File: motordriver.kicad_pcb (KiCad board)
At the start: 2 copper layers, 8 parts, among them J1 power terminal, J2 motor A, J3 motor B, J4 control pins, U1 L7805, U2 L293D

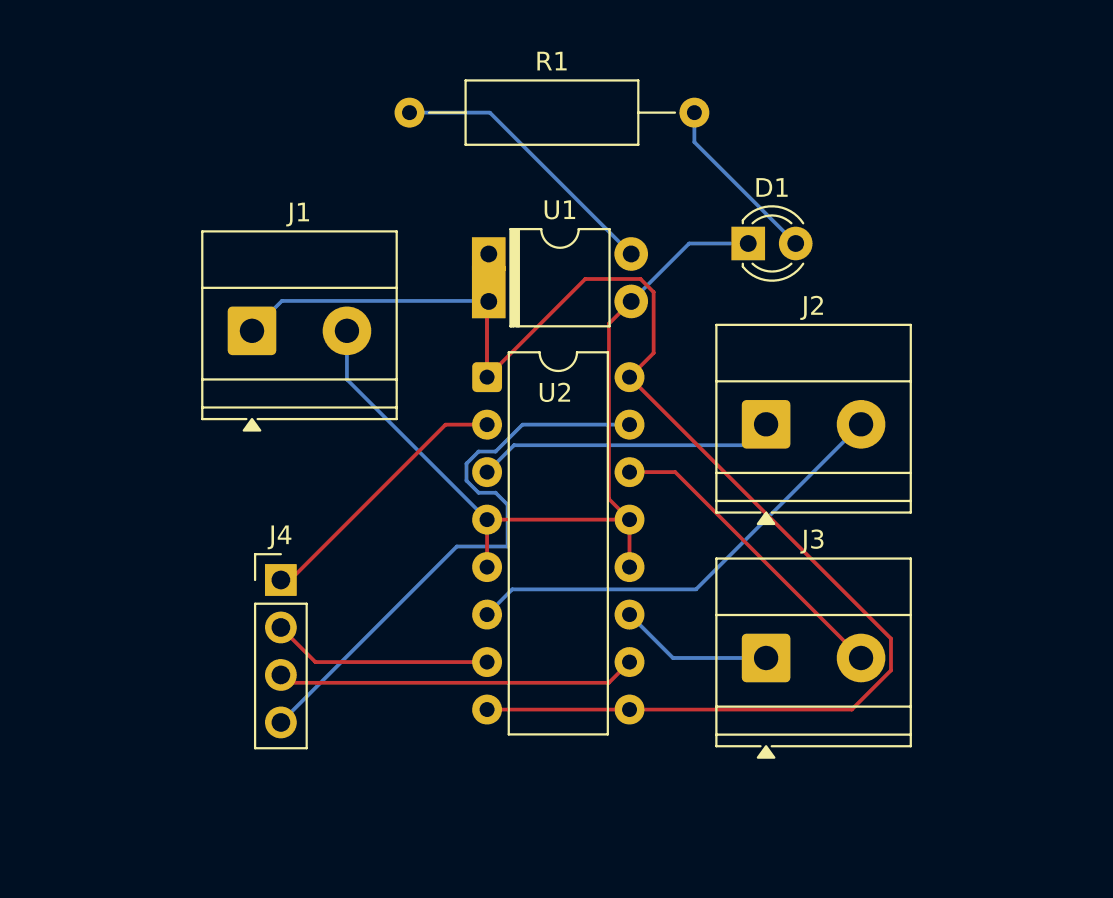
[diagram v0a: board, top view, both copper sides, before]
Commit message: done
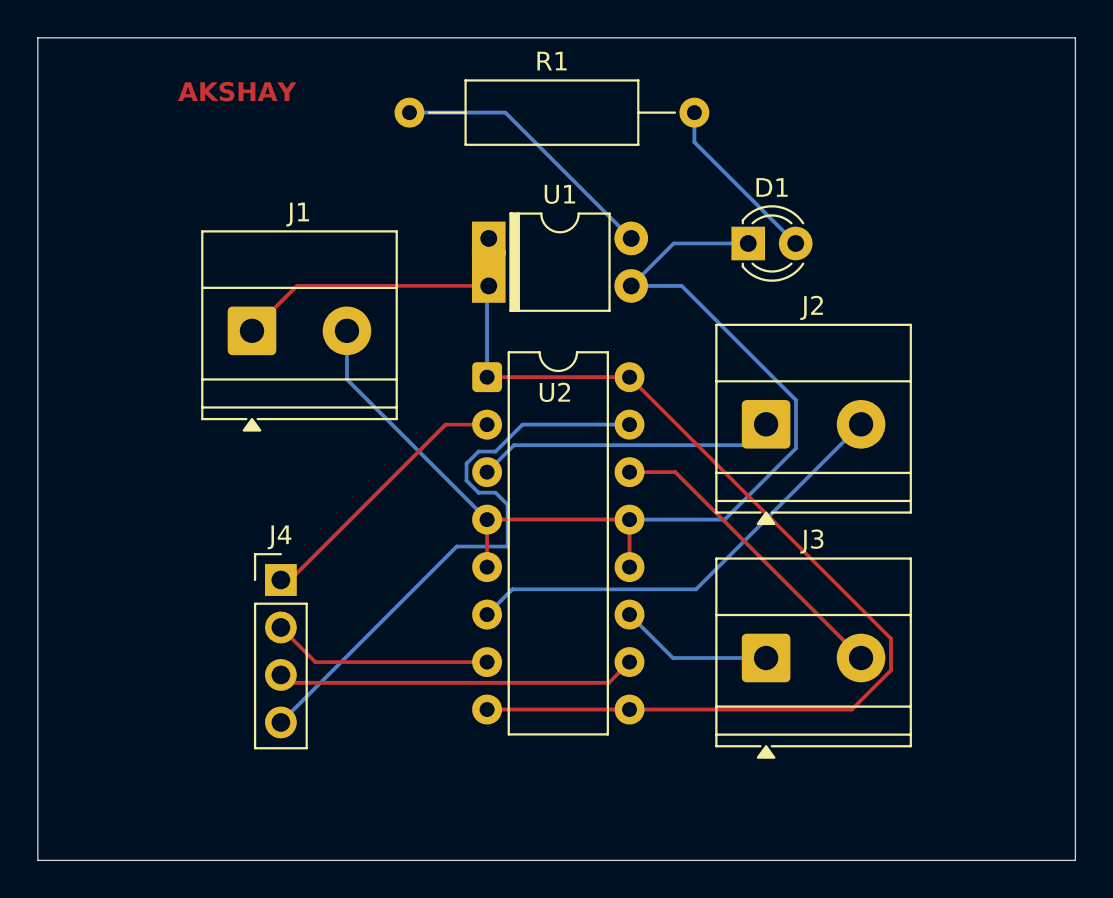
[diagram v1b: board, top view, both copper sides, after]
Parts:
- moved U1 0.83 mm to (102.1, 90.2)
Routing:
- net Net-(J1-Pin_1): track 84.5 -> 70.1 mm
- net GND: track 46.1 -> 57.5 mm
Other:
- board outline added: 55.5 x 44 mm
- board text added: "AKSHAY"
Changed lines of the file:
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@@
 	(footprint "Package_DIP:Vishay_HVM-DIP-3_W7.62mm"
 		(layer "F.Cu")
-		(at 102.12 91.06)
+		(at 102.12 90.23)
 		(descr "3-lead though-hole mounted high-volatge DIP package (based on standard DIP-4), row spacing 7.62 mm (300 mils), see https://www.vishay.com/docs/91361/hexdip.pdf")
 		(tags "THT DIP DIL PDIP 2.54mm 7.62mm 300mil Vishay HVMDIP HEXDIP")
@@
 		)
 	)
-	(segment
-		(start 108.549 94.791)
-		(end 108.549 104.169)
-		(width 0.2)
-		(layer "F.Cu")
-		(net 1)
+	(gr_rect
+		(start 78 79.5)
+		(end 133.5 123.5)
+		(stroke
+			(width 0.05)
+			(type default)
+		)
+		(fill no)
+		(layer "Edge.Cuts")
+	)
+	(gr_text "AKSHAY"
+		(at 85.5 83 0)
+		(layer "F.Cu")
+		(effects
+			(font
+				(size 1 1)
+				(thickness 0.2)
+				(bold yes)
+			)
+			(justify left bottom)
+		)
 	)
 	(segment
@@
 	)
 	(segment
-		(start 108.549 104.169)
-		(end 109.65 105.27)
-		(width 0.2)
-		(layer "F.Cu")
-		(net 1)
-	)
-	(segment
-		(start 109.74 93.6)
-		(end 108.549 94.791)
-		(width 0.2)
-		(layer "F.Cu")
-		(net 1)
-	)
-	(segment
 		(start 102.03 105.27)
 		(end 102.03 107.81)
@@
 	)
 	(segment
-		(start 109.74 93.6)
-		(end 112.84 90.5)
+		(start 109.74 92.77)
+		(end 112.01 90.5)
+		(width 0.2)
+		(layer "B.Cu")
+		(net 1)
+	)
+	(segment
+		(start 118.556 98.88734)
+		(end 118.556 101.45766)
 		(width 0.2)
 		(layer "B.Cu")
@@
 	)
 	(segment
+		(start 112.01 90.5)
+		(end 116 90.5)
+		(width 0.2)
+		(layer "B.Cu")
+		(net 1)
+	)
+	(segment
+		(start 109.74 92.77)
+		(end 112.43866 92.77)
+		(width 0.2)
+		(layer "B.Cu")
+		(net 1)
+	)
+	(segment
 		(start 94.535 95.1725)
 		(end 94.535 97.775)
@@
 	)
 	(segment
-		(start 112.84 90.5)
-		(end 116 90.5)
+		(start 112.43866 92.77)
+		(end 118.556 98.88734)
+		(width 0.2)
+		(layer "B.Cu")
+		(net 1)
+	)
+	(segment
+		(start 118.556 101.45766)
+		(end 114.74366 105.27)
+		(width 0.2)
+		(layer "B.Cu")
+		(net 1)
+	)
+	(segment
+		(start 114.74366 105.27)
+		(end 109.65 105.27)
 		(width 0.2)
 		(layer "B.Cu")
@@
 	)
 	(segment
-		(start 110.237471 92.399)
-		(end 110.941 93.102529)
-		(width 0.2)
-		(layer "F.Cu")
-		(net 3)
-	)
-	(segment
 		(start 123.636 111.636)
 		(end 123.636 113.335656)
@@
 	)
 	(segment
-		(start 110.941 93.102529)
-		(end 110.941 96.359)
-		(width 0.2)
-		(layer "F.Cu")
-		(net 3)
-	)
-	(segment
 		(start 123.636 113.335656)
 		(end 121.541656 115.43)
@@
 	)
 	(segment
-		(start 107.281 92.399)
-		(end 110.237471 92.399)
-		(width 0.2)
-		(layer "F.Cu")
-		(net 3)
-	)
-	(segment
-		(start 110.941 96.359)
-		(end 109.65 97.65)
-		(width 0.2)
-		(layer "F.Cu")
-		(net 3)
-	)
-	(segment
-		(start 102.03 97.65)
-		(end 107.281 92.399)
+		(start 89.455 95.1725)
+		(end 91.8575 92.77)
 		(width 0.2)
 		(layer "F.Cu")
@@
 	(segment
 		(start 102.03 97.65)
-		(end 102.03 91.15)
+		(end 109.65 97.65)
+		(width 0.2)
+		(layer "F.Cu")
+		(net 3)
+	)
+	(segment
+		(start 91.8575 92.77)
+		(end 102.12 92.77)
 		(width 0.2)
 		(layer "F.Cu")
@@
 	)
 	(segment
-		(start 102.03 91.15)
-		(end 102.12 91.06)
-		(width 0.2)
-		(layer "F.Cu")
+		(start 102.12 92.77)
+		(end 102.03 92.86)
+		(width 0.2)
+		(layer "B.Cu")
 		(net 3)
 	)
 	(segment
-		(start 89.455 95.1725)
-		(end 91.056 93.5715)
-		(width 0.2)
-		(layer "B.Cu")
-		(net 3)
-	)
-	(segment
-		(start 102.03 93.69)
+		(start 102.03 92.86)
 		(end 102.03 97.65)
-		(width 0.2)
-		(layer "B.Cu")
-		(net 3)
-	)
-	(segment
-		(start 102.0915 93.5715)
-		(end 102.12 93.6)
-		(width 0.2)
-		(layer "B.Cu")
-		(net 3)
-	)
-	(segment
-		(start 91.056 93.5715)
-		(end 102.0915 93.5715)
-		(width 0.2)
-		(layer "B.Cu")
-		(net 3)
-	)
-	(segment
-		(start 102.12 93.6)
-		(end 102.03 93.69)
 		(width 0.2)
 		(layer "B.Cu")
@@
 	)
 	(segment
-		(start 102.18 83.5)
-		(end 109.74 91.06)
+		(start 103.01 83.5)
+		(end 97.88 83.5)
 		(width 0.2)
 		(layer "B.Cu")
@@
 	)
 	(segment
-		(start 97.88 83.5)
-		(end 102.18 83.5)
-		(width 0.2)
-		(layer "B.Cu")
+		(start 109.74 90.23)
+		(end 103.01 83.5)
+		(width 0.2)
+		(layer "B.Cu")
